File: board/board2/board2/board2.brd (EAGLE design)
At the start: 49.5 x 45.4 mm, 9 parts

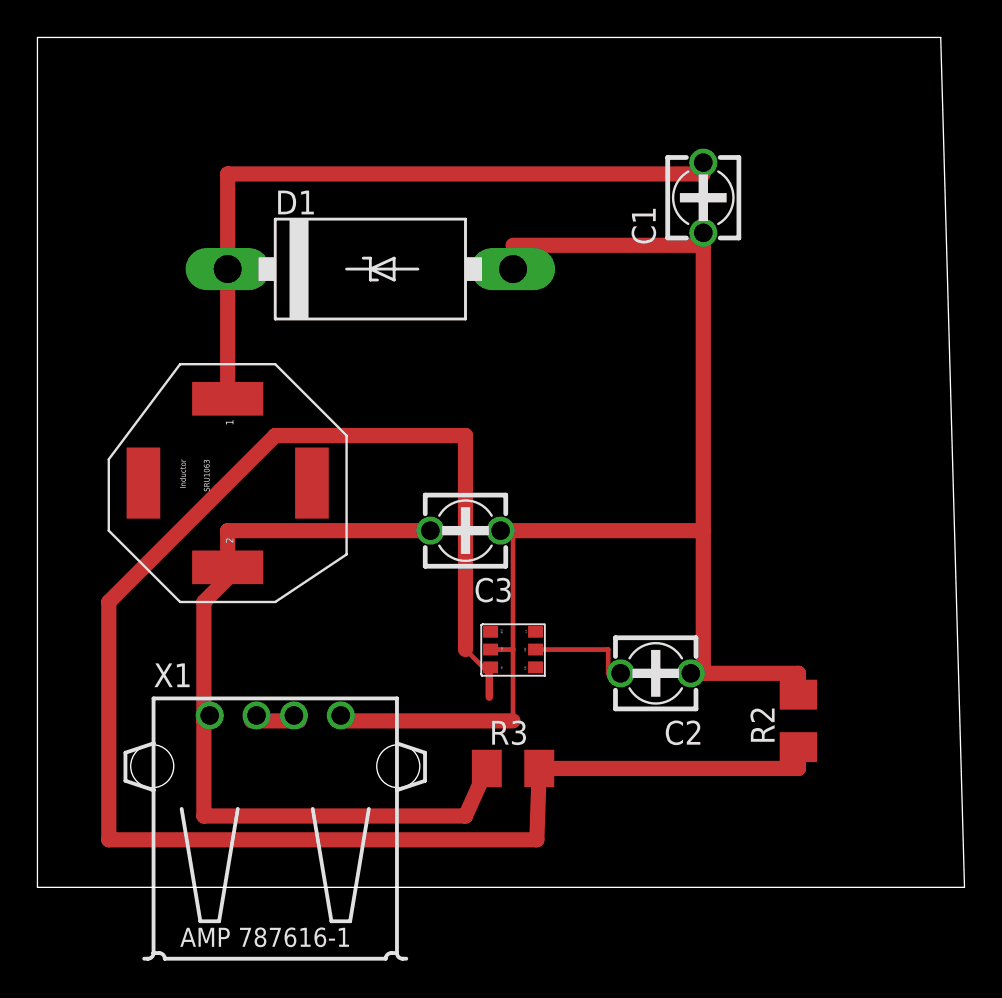
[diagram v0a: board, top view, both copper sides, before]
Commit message: updated 2nd board
need to verify junctions are all in place
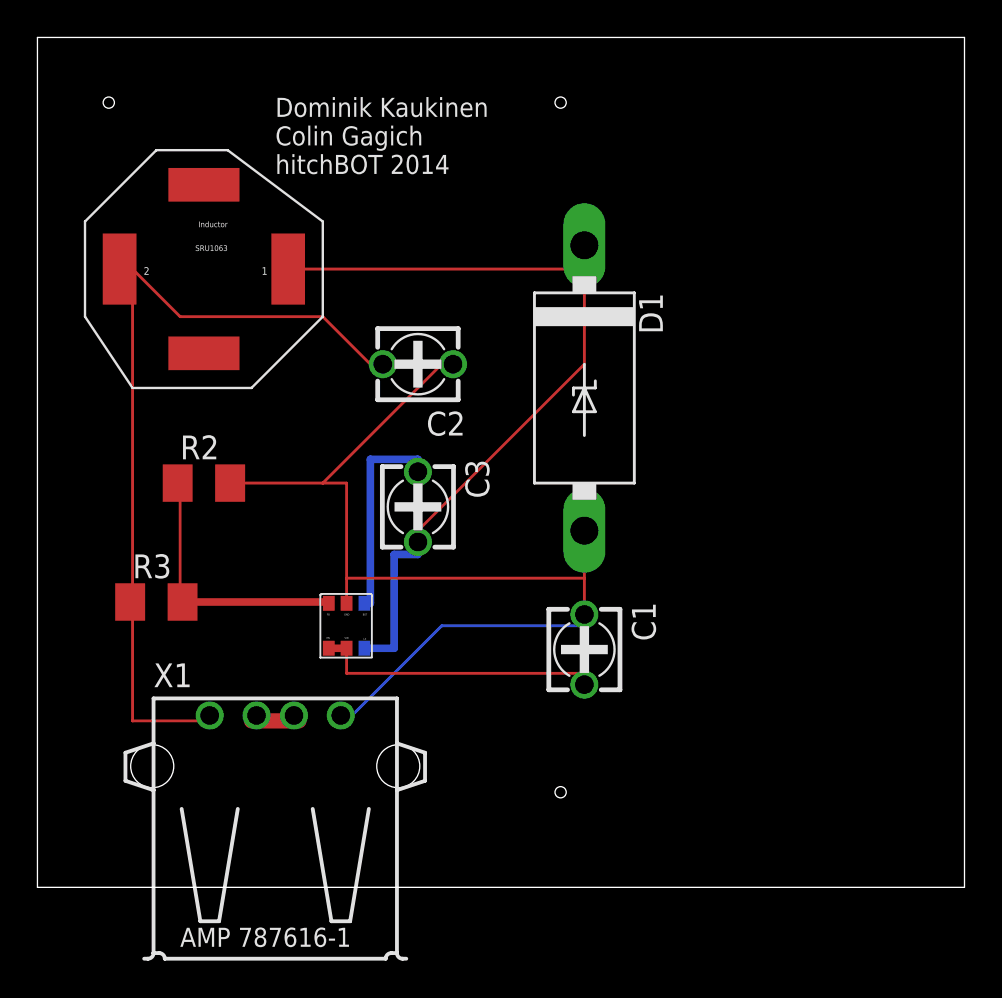
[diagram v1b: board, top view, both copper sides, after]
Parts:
- C1: value 0.1uF -> 4.7uF
- C2: value (none) -> 10uF
- C3: value (none) -> 0.1uF
- moved R2 34.2 mm to (8.89, 21.6), turned to 0 degrees
- moved C1 25.0 mm to (29.2, 12.7), turned to 270 degrees
- moved R3 21.0 mm to (6.35, 15.2)
- moved C2 20.8 mm to (20.3, 27.9)
- moved D1 13.1 mm to (29.2, 26.7), turned to 270 degrees
- moved U$2 11.5 mm to (8.89, 33.0), turned to 180 degrees
- moved U$1 8.98 mm to (16.5, 14.0), turned to 180 degrees
- moved C3 2.84 mm to (20.3, 20.3), turned to 270 degrees
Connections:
- removed net N$6: U$1.BST
- new net N$2: C3.+, U$1.BST
- net DGND: no longer C3.+
- net N$1: now also C1.-; no longer C2.-
- net N$3: now also C3.-, U$1.LX; no longer C1.-
- net N$4: now also C2.-; no longer C3.-
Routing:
- net N$5: track 92.0 -> 14.5 mm
- net DGND: track 73.4 -> 55.4 mm
- net N$2: track 0.00 -> 11.2 mm
- net N$1: track 5.81 -> 15.6 mm
- net N$3: track 38.0 -> 43.9 mm
- net N$4: track 43.8 -> 44.7 mm
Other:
- outline, holes or cut-outs redrawn
- board text added: "Dominik Kaukinen Colin Gagich hitchBOT 2014"
